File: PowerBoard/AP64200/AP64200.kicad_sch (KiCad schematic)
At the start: 52 parts, among them J1 AuxConn, J1 POWER_SW, Q10 MMBTA42, Q2 IRF9640SPBF, Q4 MMBTA92, Q6 MMBTA92, Q7 MMBTA42, Q8 MMBTA92, Q9 MMBTA92T, U5 LT8609AJDDM

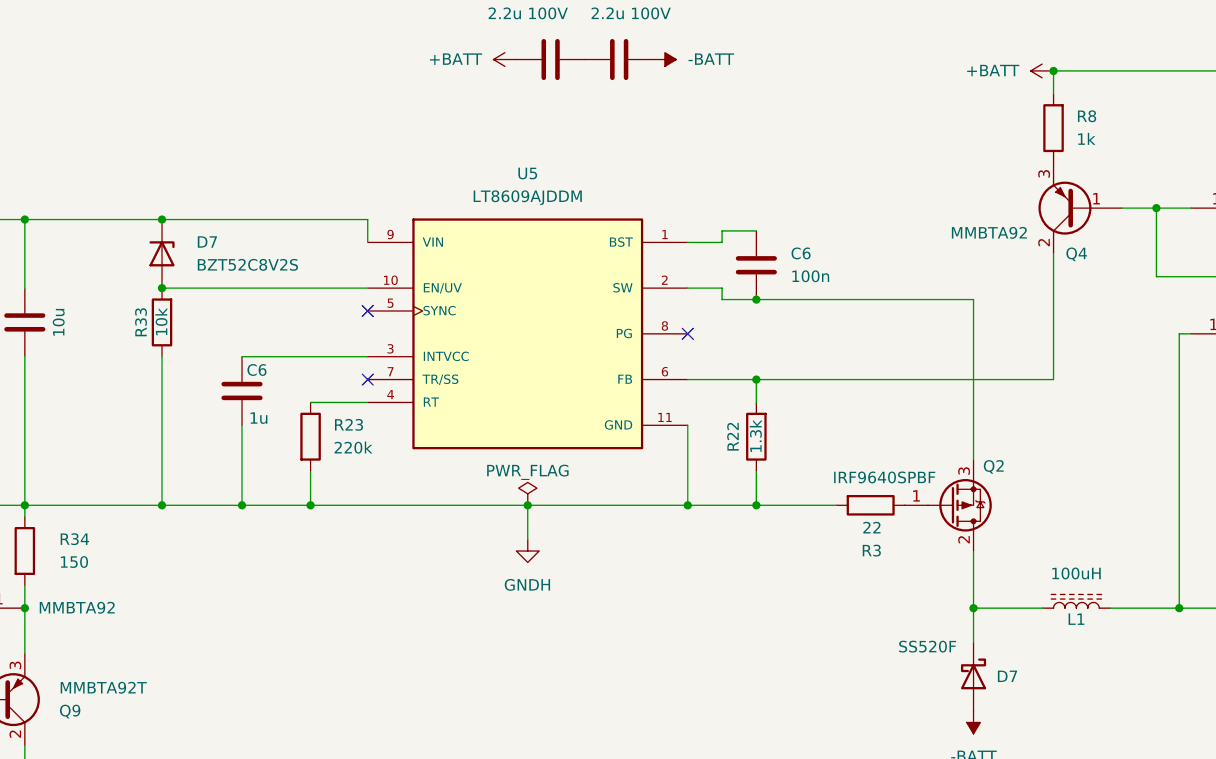
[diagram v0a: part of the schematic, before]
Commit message: v3.2.2 - TL494V2
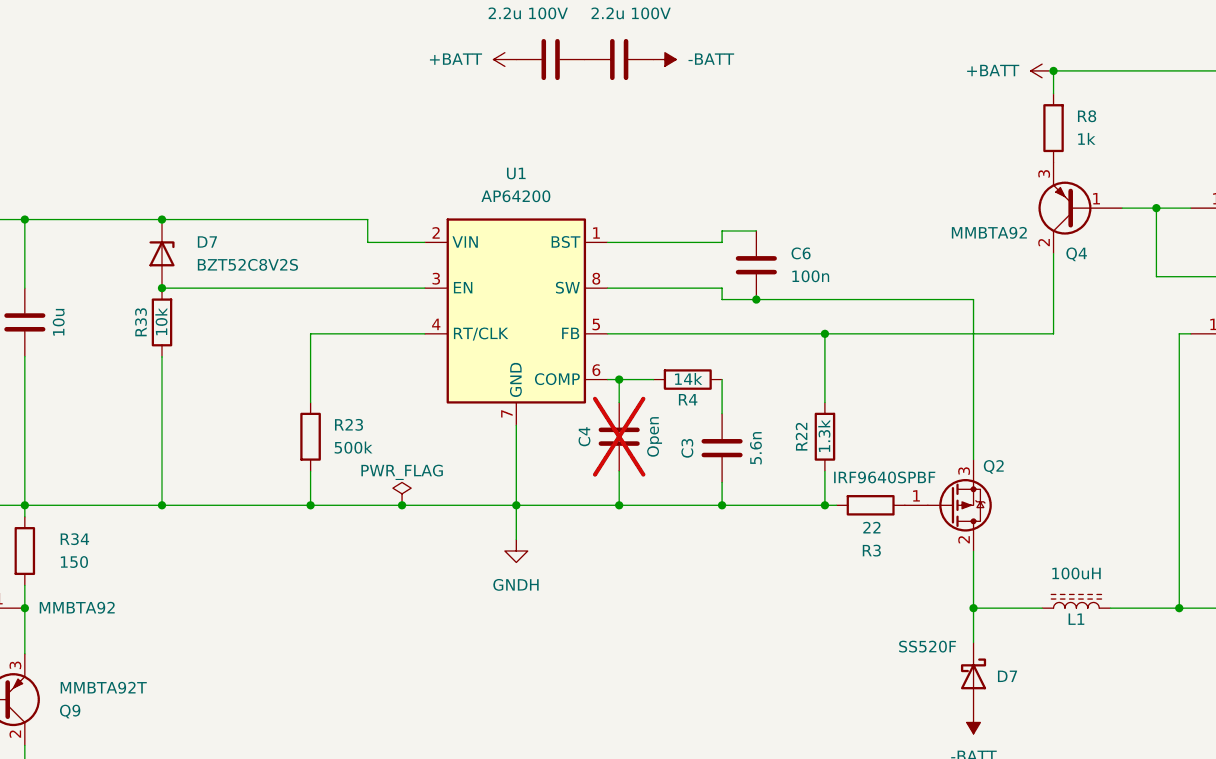
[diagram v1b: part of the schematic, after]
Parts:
- removed C6: 1u, Capacitor_SMD:C_0603_1608Metric, symbol Device:C
- removed U5: LT8609AJDDM, Package_DFN_QFN:DFN-10-1EP_2.6x2.6mm_P0.5mm_EP1.3x2.2mm, symbol GigaESCSymbols:LT8609AHDDM-5_PBF
- added C3: 5.6n, Capacitor_SMD:C_0805_2012Metric, symbol Device:C
- added C4: Open, Capacitor_SMD:C_0805_2012Metric, symbol Device:C
- added R4: 14k, Resistor_SMD:R_0603_1608Metric, symbol Device:R
- added U1: AP64200, Package_SO:SOIC-8-1EP_3.9x4.9mm_P1.27mm_EP2.62x3.51mm, symbol GigaESCSymbols:AP64200
- R23: value 220k -> 500k
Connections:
- net +BATT: now also U1.2 (VIN)
- net GNDH: now also C3.2, C4.2, U1.7 (GND), U1.9 (PAD)
- net at Q4.2 (C), R22.2: now also U1.5 (FB)
- net at C6.1, Q2.3 (S): now also U1.8 (SW)
- net at C6.2: now also U1.1 (BST)
- net at D7.2 (A), R33.2: now also U1.3 (EN)
- net at R23.1: now also U1.4 (RT/CLK)
- new net: C4.1, R4.2, U1.6 (COMP)
- new net: C3.1, R4.1
- no-connect marks 3 -> 0
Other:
- moved on the sheet: R22
